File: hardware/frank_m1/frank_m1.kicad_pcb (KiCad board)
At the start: 2 copper layers, 99.6 x 84 mm, 171 parts, among them J1 Pin Header 1x03, J10 SS-52100-004, J11 PAM L, J12 PAM R, J13 PJ-320D, J14 D-SUB 15 Female, J15 Pin Header 1x08, J16 RCA-103, J2 Pin Header 1x03, J3 USB4215-03-A, J4 MDC-036, J5 104031-0811, J6 D-SUB 9 Male, J7 D-SUB 9 Male, J8 DC3RX19JA2, J9 PJ-320D, Q1 AO3400A, Q2 AO3400A, Q3 AO3400A, Q4 AO3400A, U1 NCP1117 3.3, U10 74HC4053D,653, U11 ESP-PSRAM32, U2 PAM8403D, U3 LM358, U4 TDA1387T, U5 CD4069UBM, U6 Rasberry Pi Pico, U7 RP2040-Zero, U8 74HC4052D, U9 74HC4053D,653

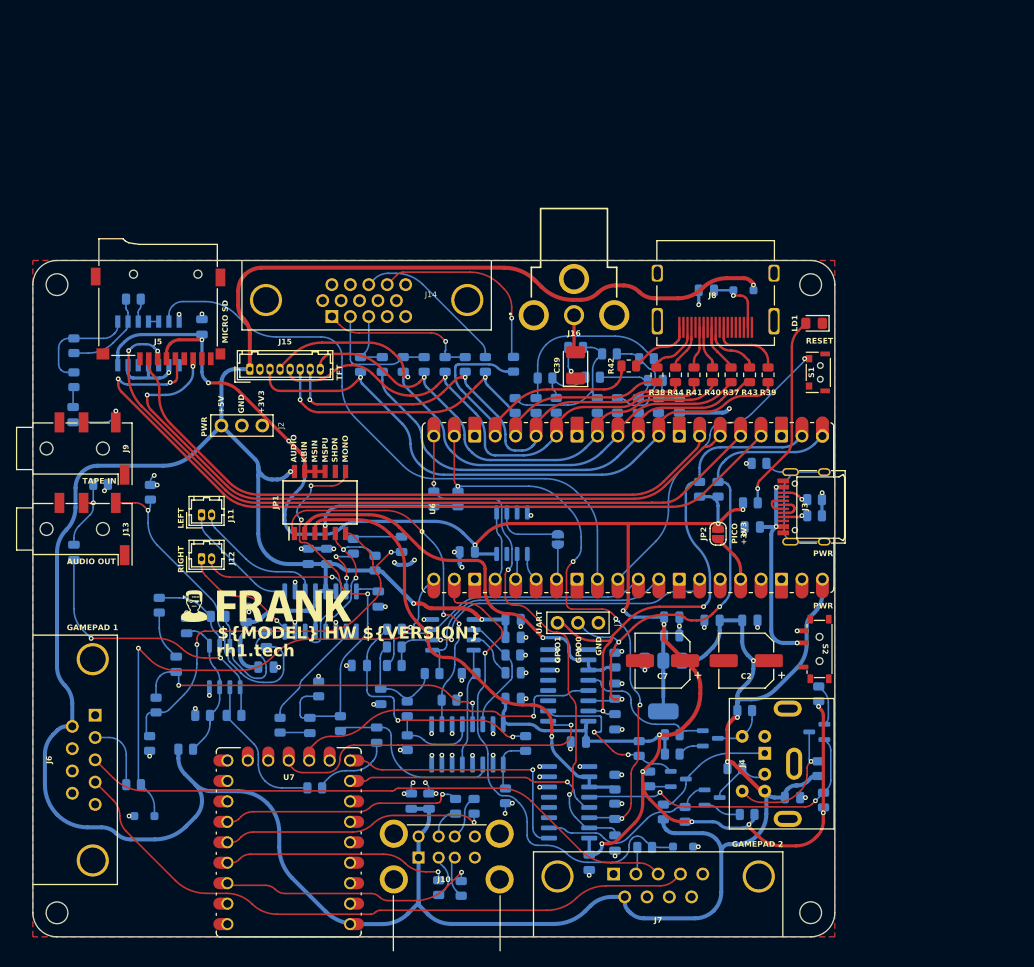
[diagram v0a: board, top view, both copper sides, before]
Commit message: New HW releases, repository cleanup
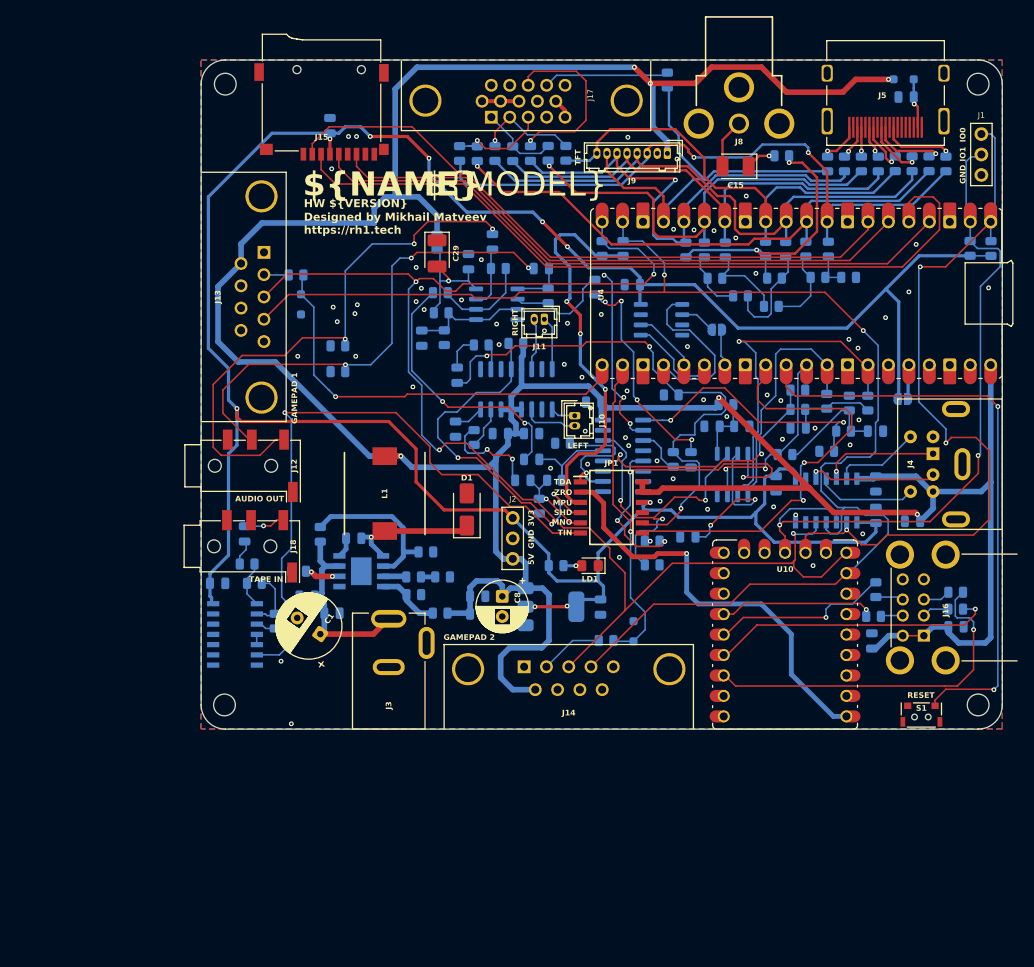
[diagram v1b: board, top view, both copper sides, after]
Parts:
- removed G***: LOGO, FRANK:FRANK Logo
- removed J6, J7: D-SUB 9 Male, FRANK:D-SUB (9 pin, male, top mount)
- removed Q1, Q2, Q3, Q4: AO3400A, FRANK:SOT-23
- removed R21, R22: 47K, FRANK:R_0805_2012Metric
- removed R65: 22K, FRANK:R_0805_2012Metric
- removed R66: 4.7K, FRANK:R_0805_2012Metric
- removed R83, R84, R85, R86: 150R, FRANK:R_0805_2012Metric
- removed R87: 51R, FRANK:R_0805_2012Metric
- removed S2: MSK12C02, FRANK:Switch (MSK12C02)
- added D4: 3V3, FRANK:Diode (SOD-323), B.Cu at (183.6, 96.0)
- added J17: D-SUB 15 Female, FRANK:D-SUB (15 pin, female), F.Cu at (165.9, 32.1)
- added J18: PJ-320D, FRANK:Jack (3.5mm, PJ-320D), F.Cu at (136.2, 85.4)
- added L1: 22uH, FRANK:CDRH104RNP, F.Cu at (152.7, 78.8)
- C1: value 100n -> 680u; footprint FRANK:C_0805_2012Metric -> FRANK:Capacitor (Radial_D8.0mm_P3.50mm); moved to F.Cu
- C10: value 1u -> 100n
- C11, C12, C13, C16, C17, C27, C3, C6: value 10u -> 100n
- C15: value 1u -> 220u; footprint FRANK:C_0805_2012Metric -> FRANK:Capacitor (3528, tantalum, polar); moved to F.Cu
- C18: value 10u -> 47n
- C19: value 100n -> 47n
- C2, C7: value 100u -> 10u; footprint FRANK:CP_Elec_6.3x5.2 -> FRANK:C_0805_2012Metric; moved to B.Cu
- C20: value 1u -> 10u
- C21: value 47u -> 100n
- C22: value 47n -> 10u
- C23: value 47n -> 1u
- C24, C26, C31, C38, C9: value 100n -> 10u
- C28, C33: value 100n -> 1u
- C29: footprint FRANK:C_0805_2012Metric -> FRANK:Capacitor (3528, tantalum, polar); moved to F.Cu
- C34: value 47pF -> 47u
- C35, C36: value 47pF -> 100n
- C37: value 47pF -> 10u
- C39: value 220u -> 100n; footprint FRANK:Capacitor (3528, tantalum, polar) -> FRANK:C_0805_2012Metric; moved to B.Cu
- C4: value 100n -> 150pF; footprint FRANK:C_0805_2012Metric -> FRANK:R_0805_2012Metric
- C8: value 100n -> 220u; footprint FRANK:C_0805_2012Metric -> FRANK:Capacitor (Radial_D6.3mm_P2.50mm); moved to F.Cu
- D1: value 3V3 -> 1N5822; footprint FRANK:Diode (SOD-323) -> FRANK:D_SMA; moved to F.Cu
- D2: value 3V3 -> 1N5819WS
- D3: value 1N5819WS -> 3V3
- J1: value Pin Header 1x03 -> UART
- J10: value SS-52100-004 -> PAM L; footprint FRANK:USB Type A (stacked) -> FRANK:Connector Female 1.25 JST 2P
- J11: value PAM L -> PAM R
- J12: value PAM R -> PJ-320D; footprint FRANK:Connector Female 1.25 JST 2P -> FRANK:Jack (3.5mm, PJ-320D)
- J13: value PJ-320D -> D-SUB 9 Male; footprint FRANK:Jack (3.5mm, PJ-320D) -> FRANK:D-SUB (9 pin, male, top mount)
- J14: value D-SUB 15 Female -> D-SUB 9 Male; footprint FRANK:D-SUB (15 pin, female) -> FRANK:D-SUB (9 pin, male, top mount)
- J15: value Pin Header 1x08 -> 104031-0811; footprint FRANK:Connector Female 1.25 JST 8P -> FRANK:MicroSD (SMD, long)
- J16: value RCA-103 -> SS-52100-004; footprint FRANK:RCJ-012 -> FRANK:USB Type A (stacked)
- J2: value Pin Header 1x03 -> PWR
- J3: value USB4215-03-A -> DC-005-5A-2.0; footprint FRANK:USB Type C -> FRANK:XKB_DC-005-5A-2.0
- J5: value 104031-0811 -> DC3RX19JA2; footprint FRANK:MicroSD (SMD, long) -> FRANK:HDMI (female)
- J8: value DC3RX19JA2 -> RCA-103; footprint FRANK:HDMI (female) -> FRANK:RCJ-012
- J9: value PJ-320D -> Pin Header 1x08; footprint FRANK:Jack (3.5mm, PJ-320D) -> FRANK:Connector Female 1.25 JST 8P
- JP2: moved to B.Cu
- LD1: value Power -> Green
- R10: value 1M -> 43K
- R12, R14: value 2K -> 270R
- R13, R15, R16, R17, R18, R19, R26, R29: value 10K -> 270R
- R23: value 10K -> 750R
- R24, R25: value 20K -> 270R
- R27, R28: value 1K -> 270R
- R30: value 2K -> 300R
- R31: value 10K -> 150R
- R32, R33, R34: value 2K -> 150R
- R35: value 1K -> 150R
- R36: value 1K -> 51R
- R37: value 270R -> 4.7K; moved to B.Cu
- R38, R39: value 270R -> 100K; moved to B.Cu
- R40, R42: value 270R -> 10K; moved to B.Cu
- R41, R43, R44: value 270R -> 2K; moved to B.Cu
- R45: value 470R -> 2K
- R46: value 470R -> 1K
- R47: value 4.7K -> 1K
- R48, R49: value 100K -> 470R
- R5, R7: value 22K -> 100K
- R50, R52: value 22K -> 2K
- R51: value 4.7K -> 10K
- R53, R54, R55, R56: value 22R -> 10K
- R57, R58: value 330R -> 10K
- R59: value 330R -> 47K
- R6: value 4.7K -> 24K
- R60: value 1K -> 47K
- R61: value 1K -> 10K
- R62: value 1K -> 20K
- R63: value 100R -> 20K
- R64: value 100R -> 10K
- R67: value 22K -> 1K
- R68: value 10K -> 1K
- R69, R70: value 10K -> 22R
- R71: value 22K -> 22R
- R72: value 4.7K -> 22R
- R73: value 22K -> 330R
- R74: value 750R -> 330R
- R75: value 270R -> 330R
- R76, R77, R78: value 270R -> 1K
- R79, R80: value 270R -> 100R
- R8: value 5.1K -> 100K
- R81: value 300R -> 100R
- R82: value 150R -> 100R
- R9: value 5.1K -> 8.2K
- U1: value NCP1117 3.3 -> MP1584EN-LF-Z; footprint FRANK:SOT-223 -> FRANK:SOIC127P600X170-9N
- U10: value 74HC4053D,653 -> RP2040-Zero; footprint FRANK:SOP-16 -> FRANK:Raspberry Pi Zero; moved to F.Cu
- U2: value PAM8403D -> AMS1117 3.3; footprint FRANK:SOP-16 -> FRANK:SOT-223
- U3: value LM358 -> TXS0104EDR; footprint FRANK:SO-8 -> FRANK:SOIC127P600X175-14N
- U4: value TDA1387T -> Rasberry Pi Pico; footprint FRANK:SO-8 -> FRANK:Raspberry Pi Pico; moved to F.Cu
- U6: value Rasberry Pi Pico -> TDA1387T; footprint FRANK:Raspberry Pi Pico -> FRANK:SO-8; moved to B.Cu
- U7: value RP2040-Zero -> PAM8403D; footprint FRANK:Raspberry Pi Zero -> FRANK:SOP-16; moved to B.Cu
- U8: value 74HC4052D -> LM358; footprint FRANK:SOP-16 -> FRANK:SO-8
- U9: value 74HC4053D,653 -> 74HC4052D
- moved R12 119.0 mm to (218.2, 37.9)
- moved R16 112.6 mm to (214.0, 37.9), turned to -90 degrees
- moved R13 108.7 mm to (209.8, 37.9)
- moved R17 103.5 mm to (207.7, 37.9), turned to -90 degrees
- moved R19 103.0 mm to (211.9, 37.9)
- moved R14 101.6 mm to (222.4, 37.9), turned to -90 degrees
- moved C18 100.7 mm to (213.7, 71.1), turned to 0 degrees
- moved D2 99.2 mm to (217.2, 27.4), turned to 180 degrees
- moved R27 99.1 mm to (195.0, 48.6), turned to -90 degrees
- moved R15 97.9 mm to (216.1, 37.9), turned to -90 degrees
- moved J5 95.3 mm to (214.9, 32.6), turned to 180 degrees
- moved C14 90.5 mm to (217.4, 29.6), turned to 180 degrees
- moved R25 90.0 mm to (202.5, 48.5), turned to -90 degrees
- moved R67 89.2 mm to (141.7, 51.7), turned to 180 degrees
- moved C11 88.8 mm to (213.7, 81.5)
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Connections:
- C1 pad 1: Net-(S2-B) -> /Power/VBUS_IN
- C10 pad 1: /MONO_L -> VBUS
- C10 pad 2: Net-(C10-Pad2) -> GND
- C11 pad 1: /AMP_L -> +3V3
- C11 pad 2: Net-(C11-Pad2) -> GND
- C12 pad 1: /AMP_R -> +3V3
- C12 pad 2: Net-(C12-Pad2) -> GND
- C13 pad 1: GND -> VBUS
- C13 pad 2: Net-(U3A-+) -> GND
- C14 pad 1: Net-(U2-VREF) -> Net-(D2-K)
- C15 pad 1: /MONO_R -> Net-(C15-Pad1)
- C15 pad 2: Net-(C15-Pad2) -> /Composite/CVBS
- C16 pad 1: GND -> Net-(C16-Pad1)
- C16 pad 2: VBUS -> /Tape In/TAPE
- C17 pad 1: Net-(C17-Pad1) -> +3V3
- C17 pad 2: /Audio/AMP_OUTL -> GND
- C18 pad 2: /Audio/AMP_OUTR -> GND
- C19 pad 1: GND -> Net-(C19-Pad1)
- C19 pad 2: VBUS -> GND
- C2 pad 1: VBUS -> /Power/VBUS_IN
- C20 pad 1: VBUS -> Net-(U6-VA)
- C21 pad 1: VBUS -> Net-(U6-VA)
- C22 pad 1: Net-(C22-Pad1) -> Net-(U6-FLT)
- C23 pad 1: Net-(C23-Pad1) -> /MONO_L
- C23 pad 2: GND -> Net-(C23-Pad2)
- C24 pad 1: Net-(D3-K) -> /AMP_L
- C24 pad 2: GND -> Net-(C24-Pad2)
- C25 pad 1: VBUS -> /AMP_R
- C25 pad 2: GND -> Net-(C25-Pad2)
- C26 pad 1: VBUS -> GND
- C26 pad 2: GND -> Net-(U8A-+)
- C27 pad 1: Net-(U4-FLT) -> Net-(U7-VREF)
- C28 pad 1: Net-(C28-Pad1) -> /MONO_R
- C28 pad 2: /Tape In/TAPE -> Net-(C28-Pad2)
- C29 pad 1: VBUS -> GND
- C29 pad 2: GND -> Net-(U8C-V+)
- C3 pad 1: VBUS -> /Power/VBUS_IN
- C30 pad 1: VBUS -> Net-(C30-Pad1)
- C30 pad 2: GND -> /AMP_OUT_L
- C31 pad 1: GND -> Net-(C31-Pad1)
- C31 pad 2: +3V3 -> /AMP_OUT_R
- C32 pad 2: +3V3 -> Net-(U8C-V+)
- C33 pad 1: GND -> VBUS
- C33 pad 2: +3V3 -> GND
- C34 pad 1: GND -> VBUS
- C34 pad 2: /PGPIO1 -> GND
- C35 pad 2: /PGPIO15 -> VBUS
- C36 pad 2: /PGPIO0 -> +3V3
- C37 pad 1: GND -> VBUS
- C37 pad 2: /PGPIO14 -> GND
- C38 pad 1: +3V3 -> VBUS
- C39 pad 1: Net-(C39-Pad1) -> +3V3
- C39 pad 2: /Composite/CVBS -> GND
- C4 pad 1: VBUS -> Net-(U1-COMP)
- C4 pad 2: GND -> Net-(C4-Pad2)
- C5 pad 1: +3V3 -> Net-(U1-BST)
- C5 pad 2: GND -> Net-(D1-K)
- C6 pad 1: +3V3 -> GND
- C6 pad 2: GND -> VBUS
- C7 pad 1: +3V3 -> VBUS
- C9 pad 1: GND -> +3V3
- C9 pad 2: +3V3 -> GND
- D1 pad 1: /PGPIO16 -> Net-(D1-K)
- D2 pad 1: /PGPIO17 -> Net-(D2-K)
- D2 pad 2: GND -> VBUS
- D3 pad 1: Net-(D3-K) -> /PGPIO16
- D3 pad 2: VBUS -> GND
- J1 pad 1: GND -> /PGPIO0
- J1 pad 2: /PGPIO0 -> /PGPIO1
- J1 pad 3: /PGPIO1 -> GND
- J10 pad 1: VBUS -> /Audio/AMP_PAM_OUTL_P
- J10 pad 2: Net-(J10-D1-) -> /Audio/AMP_PAM_OUTL_M
- J11 pad 1: /Audio/AMP_PAM_OUTL_P -> /Audio/AMP_PAM_OUTR_P
- J11 pad 2: /Audio/AMP_PAM_OUTL_M -> /Audio/AMP_PAM_OUTR_M
- J14 pad 1: Net-(J14-Pad1) -> unconnected-(J14-Pad1)
- J14 pad 3: Net-(J14-Pad3) -> /PGPIO15
- J14 pad 4: unconnected-(J14-Pad4) -> /PGPIO14
- J14 pad 5: GND -> unconnected-(J14-Pad5)
- J14 pad 6: GND -> VBUS
- J14 pad 7: GND -> unconnected-(J14-Pad7)
- J15 pad 1: VBUS -> unconnected-(J15-DAT2-Pad1)
- J15 pad 2: GND -> /PGPIO5
- J15 pad 3: /PGPIO6 -> /PGPIO3
- J15 pad 4: /PGPIO8 -> +3V3
- J15 pad 5: /PGPIO10 -> /PGPIO2
- J15 pad 6: /PGPIO12 -> GND
- J15 pad 7: /PGPIO11 -> /PGPIO4
- J15 pad 8: /PGPIO9 -> unconnected-(J15-DAT1-Pad8)
- J16 pad 1: /Composite/CVBS -> VBUS
- J16 pad 2: GND -> Net-(J16-D1-)
- J3 pad 1: GND -> /Power/VBUS_IN
- J3 pad 2: Net-(S2-B) -> GND
- J5 pad 1: unconnected-(J5-DAT2-Pad1) -> Net-(J5-D2P)
- J5 pad 2: /PGPIO5 -> GND
- J5 pad 3: /PGPIO3 -> Net-(J5-D2N)
- J5 pad 4: +3V3 -> Net-(J5-D1P)
- J5 pad 5: /PGPIO2 -> GND
- J5 pad 6: GND -> Net-(J5-D1N)
- J5 pad 7: /PGPIO4 -> Net-(J5-D0P)
- J5 pad 8: unconnected-(J5-DAT1-Pad8) -> GND
- J5 pad 9: unconnected-(J5-SHIELD-Pad9) -> Net-(J5-D0N)
- J8 pad 1: Net-(J8-D2P) -> /Composite/CVBS
- JP1 pad 1: /ASW -> /AUDIOSW
- JP1 pad 11: +3V3 -> VBUS
- JP1 pad 2: /PSW_KB -> /Z_VBUS
- JP1 pad 3: /PSW_MS -> /MSPUP3V3
- JP1 pad 4: /MSPUP3V3 -> /SHND
- JP1 pad 5: /SHND -> /MONO_L
- JP1 pad 6: /MONO_L -> /LOAD_IN
- JP1 pad 7: /MONO_R -> /PGPIO22
- JP1 pad 8: GND -> /MONO_R
- JP1 pad 9: +3V3 -> GND
- R1 pad 1: /PGPIO0 -> /PGPIO15
- R1 pad 2: +3V3 -> /MSPUP3V3
- R10 pad 1: Net-(J3-SHIELD) -> VBUS
- R10 pad 2: GND -> Net-(U1-FB)
- R12 pad 1: /MONO_L -> Net-(J5-D0N)
- R12 pad 2: GND -> /PGPIO8
- R13 pad 1: /AMP_L -> Net-(J5-D2N)
- R13 pad 2: /MONO_L -> /PGPIO12
- R14 pad 1: /MONO_R -> Net-(J5-CLKN)
- R14 pad 2: GND -> /PGPIO6
- R15 pad 1: /AMP_R -> Net-(J5-D0P)
- R15 pad 2: /MONO_R -> /PGPIO9
- R16 pad 1: Net-(U3A-+) -> Net-(J5-D1N)
- R16 pad 2: VBUS -> /PGPIO10
- R17 pad 1: GND -> Net-(J5-D2P)
- R17 pad 2: Net-(U3A-+) -> /PGPIO13
- R18 pad 1: Net-(U2-INL) -> Net-(J5-CLKP)
- R18 pad 2: Net-(C10-Pad2) -> /PGPIO7
- R19 pad 1: Net-(U3B--) -> Net-(J5-D1P)
- R19 pad 2: Net-(C11-Pad2) -> /PGPIO11
- R2 pad 1: /PGPIO1 -> /PGPIO14
- R2 pad 2: +3V3 -> /MSPUP3V3
- R20 pad 1: Net-(U3A--) -> GND
- R20 pad 2: Net-(C12-Pad2) -> /AUDIOSW
- R23 pad 1: Net-(U2-INR) -> /PGPIO12
- R23 pad 2: Net-(C15-Pad2) -> Net-(R23-Pad2)
- R24 pad 1: GND -> /PGPIO9
- R24 pad 2: /Audio/AMP_OUTL -> Net-(R23-Pad2)
- R25 pad 1: GND -> /PGPIO8
- R25 pad 2: /Audio/AMP_OUTR -> Net-(R25-Pad2)
- R26 pad 1: VBUS -> /PGPIO11
- R26 pad 2: /SHND -> Net-(R26-Pad2)
- R27 pad 1: /PGPIO16 -> /PGPIO10
- R27 pad 2: Net-(J6-Pad2) -> Net-(R27-Pad2)
- R28 pad 1: /PGPIO17 -> /PGPIO7
- R28 pad 2: Net-(J7-Pad2) -> Net-(R28-Pad2)
- R29 pad 1: Net-(C22-Pad1) -> /PGPIO6
- R29 pad 2: /PWM_R -> Net-(R29-Pad2)
- R3 pad 1: /PGPIO14 -> /PGPIO1
- R3 pad 2: /MSPUP3V3 -> +3V3
- R30 pad 1: /PWM_R -> GND
- R30 pad 2: GND -> Net-(R29-Pad2)
- R31 pad 1: Net-(C23-Pad1) -> Net-(R25-Pad2)
- R31 pad 2: /PWM_L -> Net-(R23-Pad2)
- R32 pad 1: /PWM_L -> Net-(R26-Pad2)
- R32 pad 2: GND -> Net-(R25-Pad2)
- R33 pad 1: /PGPIO28 -> Net-(R27-Pad2)
- R33 pad 2: Net-(C22-Pad1) -> Net-(R26-Pad2)
- R34 pad 1: /PGPIO28 -> Net-(R28-Pad2)
- R34 pad 2: Net-(C23-Pad1) -> Net-(R27-Pad2)
- R35 pad 1: Net-(C23-Pad1) -> Net-(R29-Pad2)
- R35 pad 2: /PGPIO27 -> Net-(R28-Pad2)
- R36 pad 1: Net-(C22-Pad1) -> Net-(R23-Pad2)
- R36 pad 2: /PGPIO26 -> Net-(C15-Pad1)
- R37 pad 1: Net-(J8-D0N) -> Net-(U5-A)
- R37 pad 2: /PGPIO8 -> Net-(C16-Pad1)
- R38 pad 1: Net-(J8-D2N) -> Net-(U5-G-*A)
- R38 pad 2: /PGPIO12 -> Net-(U5-A)
- R39 pad 1: Net-(J8-CLKN) -> Net-(U5-B)
- R39 pad 2: /PGPIO6 -> Net-(U5-G-*A)
- R4 pad 1: /PGPIO15 -> /PGPIO0
- R4 pad 2: /MSPUP3V3 -> +3V3
- R40 pad 1: Net-(J8-D0P) -> Net-(C18-Pad1)
- R40 pad 2: /PGPIO9 -> /PWM_R
- R41 pad 1: Net-(J8-D1N) -> /PWM_R
- R41 pad 2: /PGPIO10 -> GND
- R42 pad 1: Net-(J8-D2P) -> Net-(C19-Pad1)
- R42 pad 2: /PGPIO13 -> /PWM_L
- R43 pad 1: Net-(J8-CLKP) -> /PWM_L
- R43 pad 2: /PGPIO7 -> GND
- R44 pad 1: Net-(J8-D1P) -> /PGPIO28
- R44 pad 2: /PGPIO11 -> Net-(C18-Pad1)
- R45 pad 1: /TDA_R -> /PGPIO28
- R45 pad 2: GND -> Net-(C19-Pad1)
- R46 pad 1: GND -> Net-(C19-Pad1)
- R46 pad 2: /TDA_L -> /PGPIO27
- R47 pad 1: Net-(U5-A) -> Net-(C18-Pad1)
- R47 pad 2: Net-(C28-Pad1) -> /PGPIO26
- R48 pad 1: Net-(U5-G-*A) -> /TDA_R
- R48 pad 2: Net-(U5-A) -> GND
- R49 pad 1: Net-(U5-B) -> GND
- R49 pad 2: Net-(U5-G-*A) -> /TDA_L
- R5 pad 1: +3V3 -> /EN
- R5 pad 2: /PS2_K_DATA -> /Power/VBUS_IN
- R50 pad 1: +3V3 -> /MONO_L
- R50 pad 2: /PS2_M_DATA -> GND
- R51 pad 1: +3V3 -> /AMP_L
- R51 pad 2: Net-(Q2-G) -> /MONO_L
- R52 pad 1: VBUS -> /MONO_R
- R52 pad 2: /PS2/MS_DATA_5V -> GND
- R53 pad 1: /ZGPIO2 -> /AMP_R
- R53 pad 2: Net-(J10-D1+) -> /MONO_R
- R54 pad 1: /ZGPIO3 -> Net-(U8A-+)
- R54 pad 2: Net-(J10-D1-) -> Net-(U8C-V+)
- R55 pad 1: /ZGPIO4 -> GND
- R55 pad 2: Net-(J10-D2+) -> Net-(U8A-+)
- R56 pad 1: /ZGPIO5 -> Net-(U7-INL)
- R56 pad 2: Net-(J10-D2-) -> Net-(C23-Pad2)
- R57 pad 1: /PGPIO11 -> Net-(U8B--)
- R57 pad 2: Net-(J14-Pad1) -> Net-(C24-Pad2)
- R58 pad 1: /PGPIO9 -> Net-(U8A--)
- R58 pad 2: Net-(J14-Pad2) -> Net-(C25-Pad2)
- R59 pad 1: /PGPIO7 -> Net-(C30-Pad1)
- R59 pad 2: Net-(J14-Pad3) -> Net-(U8B--)
- R6 pad 1: +3V3 -> /EN
- R6 pad 2: Net-(Q1-G) -> GND
- R60 pad 1: /PGPIO10 -> Net-(C31-Pad1)
- R60 pad 2: Net-(J14-Pad1) -> Net-(U8A--)
- R61 pad 1: /PGPIO8 -> Net-(U7-INR)
- R61 pad 2: Net-(J14-Pad2) -> Net-(C28-Pad2)
- R62 pad 1: /PGPIO6 -> GND
- R62 pad 2: Net-(J14-Pad3) -> /AMP_OUT_L
- R63 pad 1: Net-(J14-Pad13) -> GND
- R63 pad 2: /PGPIO12 -> /AMP_OUT_R
- R64 pad 1: Net-(J14-Pad14) -> VBUS
- R64 pad 2: /PGPIO13 -> /SHND
- R67 pad 1: VBUS -> /PGPIO16
- R67 pad 2: /PS2/MS_CLK_5V -> Net-(J13-Pad2)
- R68 pad 1: GND -> /PGPIO17
- R68 pad 2: /ASW -> Net-(J14-Pad2)
- R69 pad 1: GND -> /ZGPIO2
- R69 pad 2: /PSW_KB -> Net-(J16-D1+)
- R7 pad 1: VBUS -> Net-(C4-Pad2)
- R7 pad 2: /PS2/KB_DATA_5V -> GND
- R70 pad 1: GND -> /ZGPIO3
- R70 pad 2: /PSW_MS -> Net-(J16-D1-)
- R71 pad 1: +3V3 -> /ZGPIO4
- R71 pad 2: /PS2_K_CLK -> Net-(J16-D2+)
- R72 pad 1: +3V3 -> /ZGPIO5
- R72 pad 2: Net-(Q4-G) -> Net-(J16-D2-)
- R73 pad 1: VBUS -> /PGPIO11
- R73 pad 2: /PS2/KB_CLK_5V -> Net-(J17-Pad1)
- R74 pad 1: /PGPIO12 -> /PGPIO9
- R74 pad 2: Net-(R74-Pad2) -> Net-(J17-Pad2)
- R75 pad 1: /PGPIO9 -> /PGPIO7
- R75 pad 2: Net-(R74-Pad2) -> Net-(J17-Pad3)
- R76 pad 1: /PGPIO8 -> /PGPIO10
- R76 pad 2: Net-(R76-Pad2) -> Net-(J17-Pad1)
- R77 pad 1: /PGPIO11 -> /PGPIO8
- R77 pad 2: Net-(R77-Pad2) -> Net-(J17-Pad2)
- R78 pad 1: /PGPIO10 -> /PGPIO6
- R78 pad 2: Net-(R78-Pad2) -> Net-(J17-Pad3)
- R79 pad 1: /PGPIO7 -> Net-(J17-Pad13)
- R79 pad 2: Net-(R79-Pad2) -> /PGPIO12
- R8 pad 1: GND -> Net-(U1-FREQ)
- R8 pad 2: Net-(J3-CC1) -> GND
- R80 pad 1: /PGPIO6 -> Net-(J17-Pad14)
- R80 pad 2: Net-(R80-Pad2) -> /PGPIO13
- R81 pad 1: GND -> VBUS
- R81 pad 2: Net-(R80-Pad2) -> Net-(U8C-V+)
- R82 pad 1: Net-(R76-Pad2) -> Net-(U6-VA)
- R82 pad 2: Net-(R74-Pad2) -> VBUS
- R9 pad 2: Net-(J3-CC2) -> Net-(U1-FB)
- U1 pad 1: GND -> Net-(D1-K)
- U1 pad 2: +3V3 -> /EN
- U1 pad 3: VBUS -> Net-(U1-COMP)
- U10 pad 1: /ZGPIO14 -> /ZGPIO0_1
- U10 pad 10: /PSW_MS -> /ZGPIO9_1
- U10 pad 11: /PSW_MS -> /ZGPIO10_1
- U10 pad 12: /PS2_M_CLK -> /PGPIO1
- U10 pad 13: /ZGPIO15 -> /PGPIO0
- U10 pad 14: /PGPIO14 -> /ZGPIO13_1
- U10 pad 16: +3V3 -> /PGPIO14
- U10 pad 2: /PS2_M_DATA -> /ZGPIO1_1
- U10 pad 3: unconnected-(U10-3Y1-Pad3) -> /ZGPIO2
- U10 pad 4: unconnected-(U10-3Z-Pad4) -> /ZGPIO3
- U10 pad 5: unconnected-(U10-3Y0-Pad5) -> /ZGPIO4
- U10 pad 6: GND -> /ZGPIO5
- U10 pad 7: GND -> /ZGPIO6_1
- U10 pad 8: GND -> /ZGPIO7
- U10 pad 9: GND -> /ZGPIO8
- U2 pad 1: /Audio/AMP_PAM_OUTL_P -> GND
- U2 pad 2: GND -> +3V3
- U2 pad 3: /Audio/AMP_PAM_OUTL_M -> VBUS
- U3 pad 1: Net-(C18-Pad1) -> +3V3
- U3 pad 2: Net-(U3A--) -> /PGPIO0
- U3 pad 3: Net-(U3A-+) -> /PGPIO1
- U3 pad 4: GND -> /PGPIO14
- U3 pad 5: Net-(U3A-+) -> /PGPIO15
- U3 pad 6: Net-(U3B--) -> unconnected-(U3-NC_1-Pad6)
- U3 pad 7: Net-(C17-Pad1) -> GND
- U3 pad 8: VBUS -> +3V3
- U4 pad 1: /PGPIO27 -> /PGPIO0
- U4 pad 2: /PGPIO28 -> /PGPIO1
- U4 pad 3: /PGPIO26 -> GND
- U4 pad 4: GND -> /PGPIO2
- U4 pad 5: VBUS -> /PGPIO3
- U4 pad 6: /TDA_L -> /PGPIO4
- U4 pad 7: Net-(U4-FLT) -> /PGPIO5
- U4 pad 8: /TDA_R -> GND
- U5 pad 6: /PGPIO22 -> /LOAD_IN
- U6 pad 1: /PGPIO0 -> /PGPIO27
- U6 pad 2: /PGPIO1 -> /PGPIO28
- U6 pad 3: GND -> /PGPIO26
- U6 pad 4: /PGPIO2 -> GND
- U6 pad 5: /PGPIO3 -> Net-(U6-VA)
- U6 pad 6: /PGPIO4 -> /TDA_L
- U6 pad 7: /PGPIO5 -> Net-(U6-FLT)
- U6 pad 8: GND -> /TDA_R
- U7 pad 1: /ZGPIO0 -> /Audio/AMP_PAM_OUTL_P
- U7 pad 10: /ZGPIO9 -> Net-(U7-INR)
- U7 pad 11: /ZGPIO10_1 -> GND
- U7 pad 12: /ZGPIO11 -> /SHND
- U7 pad 13: /ZGPIO12 -> VBUS
- U7 pad 14: /ZGPIO13 -> /Audio/AMP_PAM_OUTR_M
- U7 pad 15: /ZGPIO14 -> GND
- U7 pad 16: /ZGPIO15 -> /Audio/AMP_PAM_OUTR_P
- U7 pad 2: /ZGPIO1 -> GND
- U7 pad 3: /ZGPIO2 -> /Audio/AMP_PAM_OUTL_M
- U7 pad 4: /ZGPIO3 -> VBUS
- U7 pad 5: /ZGPIO4 -> VBUS
- U7 pad 6: /ZGPIO5 -> VBUS
- U7 pad 7: /ZGPIO6_1 -> Net-(U7-INL)
- U7 pad 8: /ZGPIO7 -> Net-(U7-VREF)
- U7 pad 9: /ZGPIO8_1 -> unconnected-(U7-NC-Pad9)
- U8 pad 1: /PWM_R -> Net-(C31-Pad1)
- U8 pad 2: GND -> Net-(U8A--)
- U8 pad 3: /AMP_R -> Net-(U8A-+)
- U8 pad 5: /TDA_R -> Net-(U8A-+)
- U8 pad 6: GND -> Net-(U8B--)
- U8 pad 7: GND -> Net-(C30-Pad1)
- U8 pad 8: GND -> Net-(U8C-V+)
- U9 pad 1: /ZGPIO11 -> /PWM_R
- U9 pad 10: /PSW_KB -> /AUDIOSW
- U9 pad 11: /PSW_KB -> GND
- U9 pad 12: /PS2_K_CLK -> /PWM_L
- U9 pad 13: /ZGPIO12 -> /AMP_L
- U9 pad 14: /PGPIO0 -> /TDA_L
- U9 pad 15: /PGPIO1 -> GND
- U9 pad 16: +3V3 -> VBUS
- U9 pad 2: /PS2_K_DATA -> GND
- U9 pad 3: unconnected-(U9-3Y1-Pad3) -> /AMP_R
- U9 pad 4: unconnected-(U9-3Z-Pad4) -> GND
- U9 pad 5: unconnected-(U9-3Y0-Pad5) -> /TDA_R
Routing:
- net /PGPIO14: track 70.4 -> 177.9 mm, vias 5 -> 2
- net /PGPIO15: track 65.9 -> 171.4 mm, vias 3 -> 4
- net /GAMEPAD_J4: track 81.2 -> 0.00 mm
- net /LOAD_IN: track 0.00 -> 78.2 mm, vias 0 -> 1
- net /GAMEPAD_J3: track 75.1 -> 0.00 mm
- net /AMP_OUT_L: track 0.00 -> 68.4 mm, vias 0 -> 3
- net /AMP_OUT_R: track 0.00 -> 59.0 mm, vias 0 -> 3
- net /PSW_MS: track 57.4 -> 0.00 mm, vias 1 -> 0
- net +3V3: track 262.1 -> 318.7 mm, vias 15 -> 9
- net /Z_VBUS: track 0.00 -> 52.4 mm, vias 0 -> 1
- net /PSW_KB: track 49.2 -> 0.00 mm, vias 1 -> 0
- net /ASW: track 45.6 -> 0.00 mm, vias 3 -> 0
- net VBUS: track 455.6 -> 411.3 mm, vias 8 -> 6
- net /MONO_L: track 53.4 -> 9.65 mm, vias 2 -> 1
- net /ZGPIO11: track 42.1 -> 0.00 mm, vias 1 -> 0
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- added copper zone on B.Cu, net GND
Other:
- board size 99.6 x 84 mm -> 99.5 x 83.1 mm
- board text added: "${MODEL}"
- board text added: "${NAME}"
- board text added: "3V3"
- board text added: "5V"
- board text added: "Designed by Mikhail Matveev https://rh1.tech"
- board text added: "HW ${VERSION}"
- board text added: "IO0"
- board text added: "IO1"
- board text added: "MNO"
- board text added: "MPU"
- board text added: "SHD"
- board text added: "TDA"
- board text added: "TIN"
- board text added: "ZRO"
- board text removed: "${MODEL} HW ${VERSION}"
- board text removed: "+3V3"
- board text removed: "+5V"
- board text removed: "AUDIO"
- board text removed: "GPIO0"
- board text removed: "GPIO1"
- board text removed: "KBIN"
- board text removed: "MICRO SD"
- board text removed: "MONO"
- board text removed: "MSIN"
- board text removed: "MSPU"
- board text removed: "PICO +3V3"
- board text removed: "PSRAM ENABLE"
- board text removed: "PWR"
- board text removed: "SHDN"
- board text removed: "UART"
- board text removed: "rh1.tech"
